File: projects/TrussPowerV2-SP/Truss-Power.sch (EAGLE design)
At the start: 20 parts, among them J1 XF2L-0535-1, U2 MCP73831T-2ACI/OT, U3 MAX17044, X1 22-23-2021, X2 MicroB, X3 22-23-2021

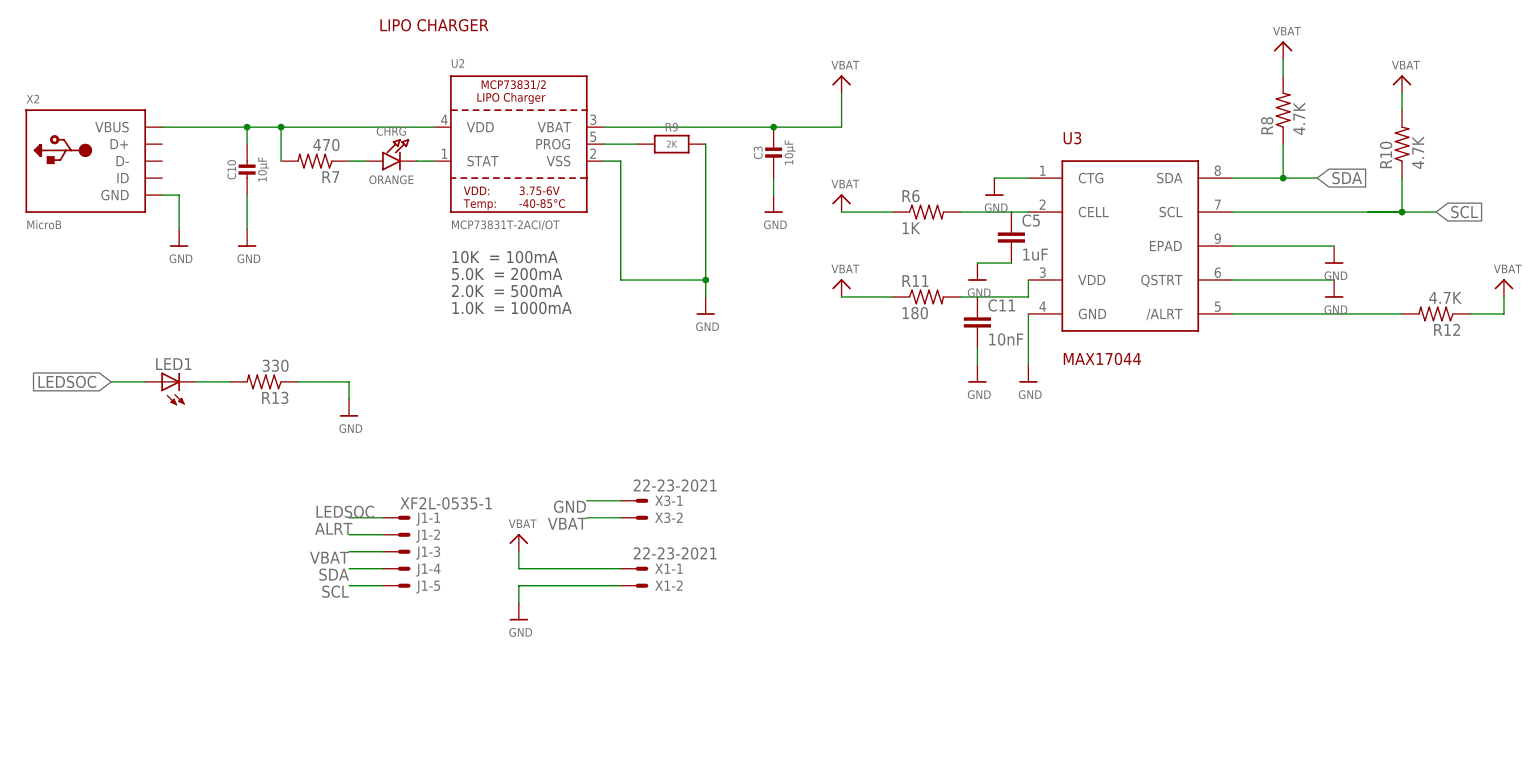
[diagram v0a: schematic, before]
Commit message: Seeedstudio
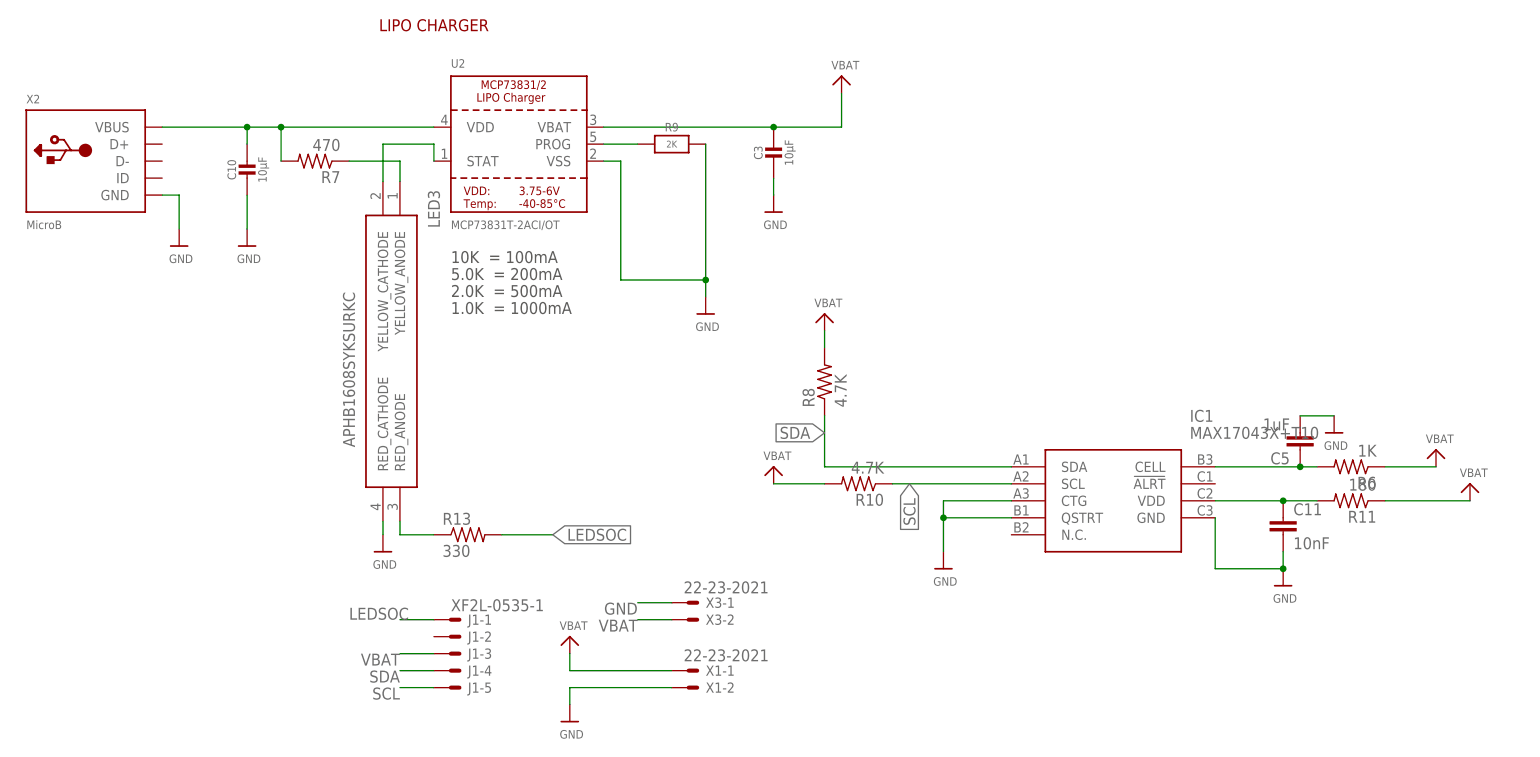
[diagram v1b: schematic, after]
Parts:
- removed CHRG: ORANGE, microbuilder:LED0805_NOOUTLINE
- removed LED1: (no value), led:LEDCHIP-LED0603
- removed R12: 4.7K, resistor:R-US_R0402
- removed U3: MAX17044, NewPart:MAX17044
- added IC1: MAX17043X+T10, SamacSys_Parts:MAX17043X+T10
- added LED3: APHB1608SYKSURKC, APHB1608SYKSURKC:APHB1608SYKSURKC
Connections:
- removed net ALRT: J1-2.MS, R12.2, U3./ALRT
- net GND: now also IC1.CTG, IC1.GND, IC1.QSTRT, LED3.RED_CATHODE; no longer R13.1, U3.CTG, U3.EPAD, U3.GND, U3.QSTRT
- net LEDSOC: now also R13.2; no longer LED1.A
- net N$1: now also IC1.CELL; no longer U3.CELL
- net N$3: now also IC1.VDD; no longer U3.VDD
- net N$4: now also LED3.YELLOW_ANODE, R7.1; no longer LED1.C, R13.2
- net N$5: now also LED3.YELLOW_CATHODE, U2.STAT; no longer CHRG.A, R7.1
- net N$6: now also LED3.RED_ANODE, R13.1; no longer CHRG.C, U2.STAT
- net SCL: now also IC1.SCL; no longer U3.SCL
- net SDA: now also IC1.SDA; no longer U3.SDA
- net VBAT: no longer R12.1
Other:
- moved on the sheet: C11, C5, J1-1, J1-2, J1-3, J1-4, J1-5, R10, R11, R13, R6, R8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
